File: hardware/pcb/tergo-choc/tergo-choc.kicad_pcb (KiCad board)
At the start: 2 copper layers, 161 x 108.8 mm, 131 parts, among them J1 TRRS, J2 Conn_01x04_Socket, J3 Conn_01x04_Socket, Q1 FDN335N, SW1 SW_Push, SW10 SW_Push, SW11 SW_Push, SW12 SW_Push, SW13 SW_Push, SW14 SW_Push, SW15 SW_Push, SW16 SW_Push, SW17 SW_Push, SW18 SW_Push, SW19 SW_Push, SW2 SW_Push, SW20 SW_Push, SW21 SW_Push, SW22 SW_Push, SW23 SW_Push, SW24 SW_Push, SW25 SW_Push, SW26 SW_Push, SW27 SW_Push, SW28 SW_Push, SW29 SW_Push, SW3 SW_Push, SW4 SW_Push, SW5 SW_Push, SW6 SW_Push, SW7 SW_Push, SW8 SW_Push, SW9 SW_Push, U1 Raspberry_Pi_Pico

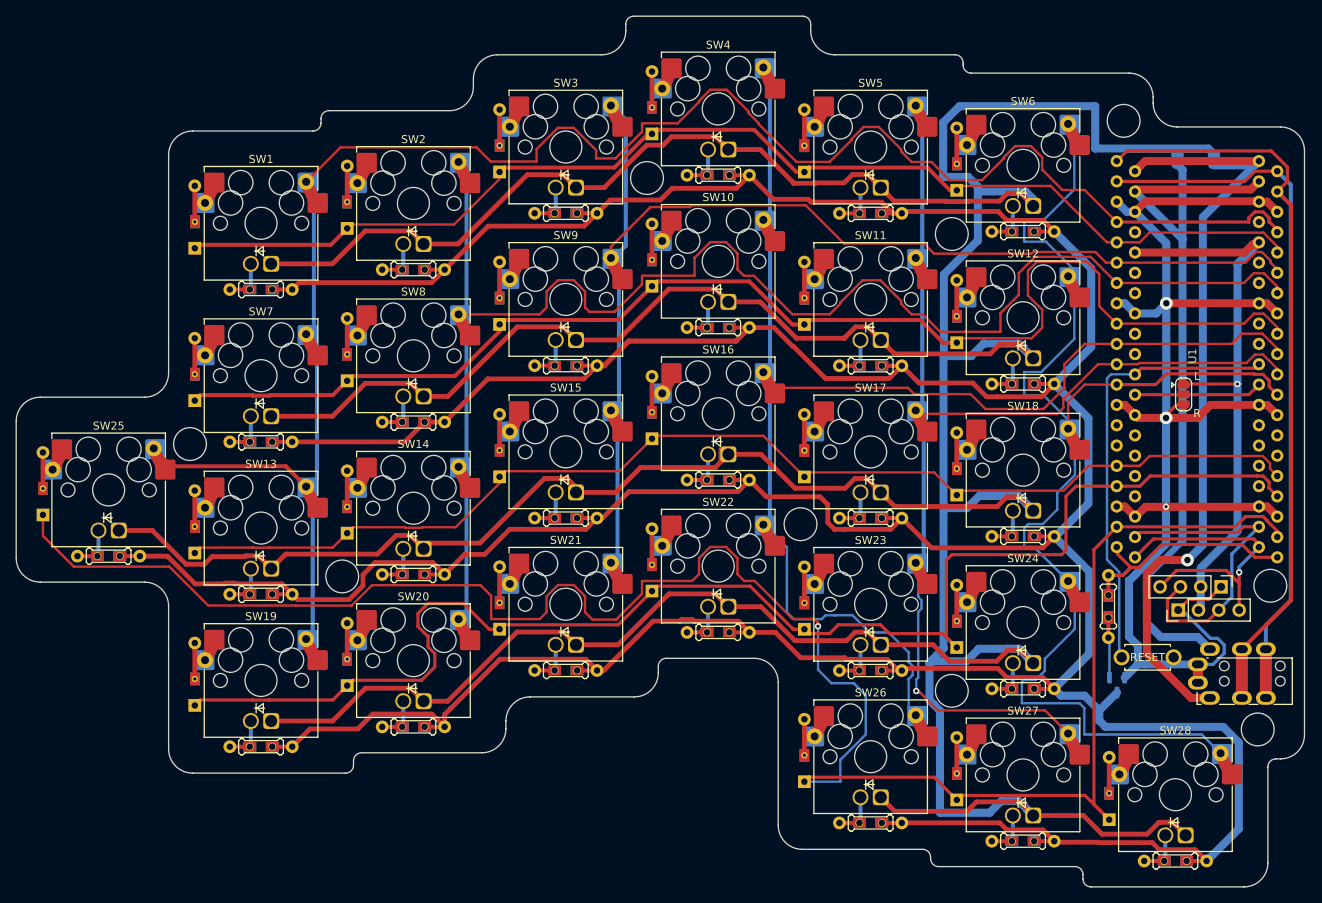
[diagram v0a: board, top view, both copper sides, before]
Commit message: wip
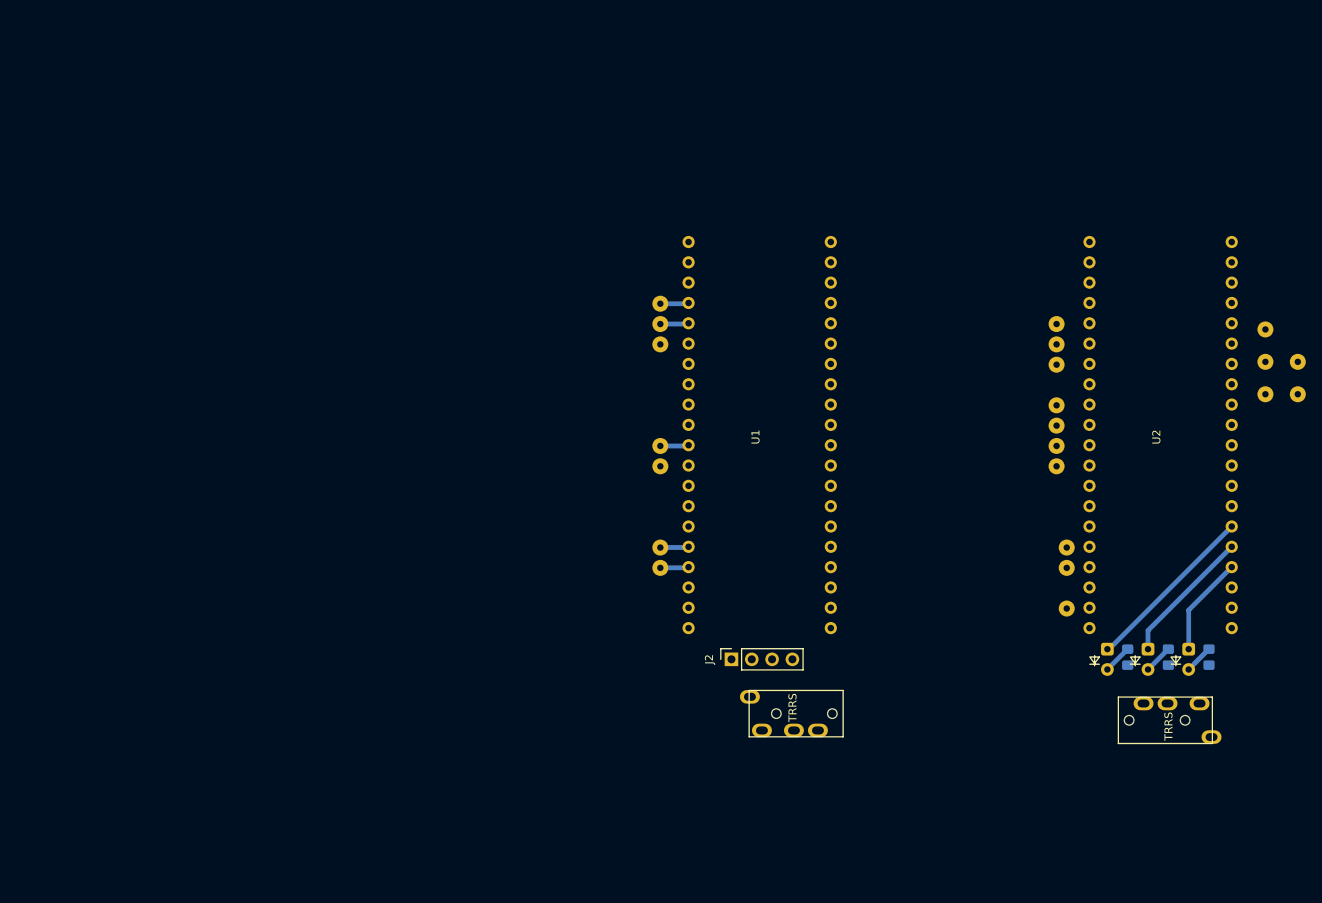
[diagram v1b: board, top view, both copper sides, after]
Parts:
- removed D1, D11, D12, D13, D14, D15, D16, D17, D18, D19, D2, D20, D21, D22, D23, D24, D25, D26, D27, D28, D3, D4, D5, D6, D7, D8, D9: D_Small, _tergo_lib:Diode-Hybrid-2sided
- removed D29, D30, D31, D32, D33, D34, D35, D36, D37, D38, D39, D40, D41, D42, D43, D44, D45, D46, D47, D48, D49, D50, D51, D52, D53, D54, D55, D56: LED_Small, _tergo_lib:LED_1.8mm
- removed H1, H2, H3, H4, H5, H6, H7, H8, H9: CaseHole, _tergo_lib:MountHole
- removed JP1: Jumper_3_Open, Jumper:SolderJumper-3_P1.3mm_Open_RoundedPad1.0x1.5mm
- removed JPL1, JPR2: Jumper_2_Open, Jumper:SolderJumper-2_P1.3mm_Open_RoundedPad1.0x1.5mm
- removed Q1: FDN335N, Package_TO_SOT_SMD:SOT-23
- removed R10, R11, R12, R13, R14, R15, R16, R17, R18, R19, R2, R20, R21, R22, R23, R24, R25, R26, R27, R28, R5, R6, R7, R8, R9: R_Small, _tergo_lib:Resistor-Hybrid-2sided
- removed R31: 10k, _tergo_lib:Resistor-Hybrid-2sided
- removed SW1, SW10, SW11, SW12, SW13, SW14, SW15, SW16, SW17, SW18, SW19, SW2, SW20, SW21, SW22, SW23, SW24, SW25, SW26, SW27, SW28, SW3, SW4, SW5, SW6, SW7, SW8, SW9: SW_Push, _tergo_lib:SW_Hotswap_Kailh_MX_Plated_mirrored2_1.00u
- removed SW29: SW_Push, _tergo_lib:ResetSW
- added D59: CL, _tergo_lib:LED_1.8mm, F.Cu at (184.2, 105.4)
- added D60: SL, _tergo_lib:LED_1.8mm, F.Cu at (189.2, 105.4)
- added J12: Conn_01x01_Socket, _tergo_lib:THT_PAD, F.Cu at (123.2, 61.0)
- added J13: Conn_01x01_Socket, _tergo_lib:THT_PAD, F.Cu at (123.2, 63.5)
- added J14: Conn_01x01_Socket, _tergo_lib:THT_PAD, F.Cu at (123.2, 66.0)
- added J15: Conn_01x01_Socket, _tergo_lib:THT_PAD, F.Cu at (198.8, 64.2)
- added J18: Conn_01x01_Socket, _tergo_lib:THT_PAD, F.Cu at (198.8, 68.2)
- added J19: Conn_01x01_Socket, _tergo_lib:THT_PAD, F.Cu at (198.8, 72.3)
- added J20: Conn_01x01_Socket, _tergo_lib:THT_PAD, F.Cu at (123.2, 78.7)
- added J21: Conn_01x01_Socket, _tergo_lib:THT_PAD, F.Cu at (123.2, 81.3)
- added J22: Conn_01x01_Socket, _tergo_lib:THT_PAD, F.Cu at (123.2, 91.4)
- added J23: Conn_01x01_Socket, _tergo_lib:THT_PAD, F.Cu at (123.2, 94.0)
- added J24: Conn_01x01_Socket, _tergo_lib:THT_PAD, F.Cu at (202.9, 68.2)
- added J25: Conn_01x01_Socket, _tergo_lib:THT_PAD, F.Cu at (202.9, 72.3)
- added J26: Conn_01x01_Socket, _tergo_lib:THT_PAD, F.Cu at (172.7, 63.5)
- added J27: Conn_01x01_Socket, _tergo_lib:THT_PAD, F.Cu at (172.7, 66.0)
- added J28: Conn_01x01_Socket, _tergo_lib:THT_PAD, F.Cu at (172.7, 68.6)
- added J29: Conn_01x01_Socket, _tergo_lib:THT_PAD, F.Cu at (172.7, 73.7)
- added J30: Conn_01x01_Socket, _tergo_lib:THT_PAD, F.Cu at (172.7, 76.2)
- added J31: Conn_01x01_Socket, _tergo_lib:THT_PAD, F.Cu at (172.7, 78.7)
- added J32: Conn_01x01_Socket, _tergo_lib:THT_PAD, F.Cu at (172.7, 81.3)
- added J33: Conn_01x01_Socket, _tergo_lib:THT_PAD, F.Cu at (174.0, 91.4)
- added J34: Conn_01x01_Socket, _tergo_lib:THT_PAD, F.Cu at (174.0, 94.0)
- added J35: Conn_01x01_Socket, _tergo_lib:THT_PAD, F.Cu at (174.0, 99.1)
- added U2: Raspberry_Pi_Pico, _tergo_lib:Raspberry_Pi_Pico, F.Cu at (185.7, 77.4)
- D10: value D_Small -> NL; footprint _tergo_lib:Diode-Hybrid-2sided -> _tergo_lib:LED_1.8mm
- J1: value TRRS -> TRRS_SOCKET; footprint _tergo_lib:MJ-4PP-9-mirrored -> _tergo_lib:MJ-4PP-9
- J2: footprint Connector_PinHeader_2.54mm:PinHeader_1x04_P2.54mm_Vertical -> Connector_PinSocket_2.54mm:PinSocket_1x04_P2.54mm_Vertical
- J3: value Conn_01x04_Socket -> TRRS_SOCKET; footprint Connector_PinHeader_2.54mm:PinHeader_1x04_P2.54mm_Vertical -> _tergo_lib:MJ-4PP-9
- R1, R3, R4: footprint _tergo_lib:Resistor-Hybrid-2sided -> Resistor_SMD:R_0805_2012Metric_Pad1.20x1.40mm_HandSolder; moved to B.Cu
- U1: footprint _tergo_lib:Raspberry_Pi_Pico_dual -> _tergo_lib:Raspberry_Pi_Pico
- moved R1 117.7 mm to (181.6, 105.1), turned to -90 degrees
- moved R3 93.5 mm to (186.7, 105.1), turned to -90 degrees
- moved R4 86.0 mm to (191.8, 105.1), turned to -90 degrees
- moved D10 76.1 mm to (179.1, 105.4), turned to 90 degrees
- moved J2 61.9 mm to (132.1, 105.4), turned to 90 degrees
- moved J1 56.1 mm to (146.2, 112.2)
- moved U1 54.5 mm to (135.6, 77.4)
- moved J3 15.8 mm to (180.3, 113.0)
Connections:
- D10 pad 1: /rowB -> Net-(D10-K)
- D10 pad 2: Net-(D10-A) -> /NUM_LOCK
- J1 pad B: /RX -> /VOUT_L
- J1 pad C: /TX -> /TX_L
- J2 pad 2: /3V3 -> /3V3_L
- R1 pad 1: Net-(D29-K) -> Net-(D10-K)
- R1 pad 2: /LEDOut -> GND
- R3 pad 2: /LEDOut -> GND
- R4 pad 2: /LEDOut -> GND
- U1 pad 10: /col3 -> /COL3_L
- U1 pad 11: /col4 -> /COL4_L
- U1 pad 12: /col5 -> /COL5_L
- U1 pad 16: /rowC -> /ROWC_L
- U1 pad 17: /rowD -> /ROWD_L
- U1 pad 19: /rowE -> /ROWE_L
- U1 pad 20: /LED -> unconnected-(U1-GP15-Pad20)
- U1 pad 29: Net-(JP1-C) -> /3V3_L
- U1 pad 30: /RST -> /RST_L
- U1 pad 36: /3V3 -> /3V3_L
- U1 pad 39: /Vin -> unconnected-(U1-Vin-Pad39)
- U1 pad 4: /col0 -> /COL0_L
- U1 pad 40: /Vout -> /VOUT_L
- U1 pad 5: /rowA -> /ROWA_L
- U1 pad 6: /col2 -> /COL2_L
- U1 pad 7: /col1 -> /COL1_L
- U1 pad 9: /rowB -> /ROWB_L
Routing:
- net /VCC_LED: track 698.5 -> 0.00 mm
- net /LEDOut: track 606.2 -> 0.00 mm
- net /rowE: track 255.9 -> 0.00 mm, vias 1 -> 0
- net /col0: track 230.9 -> 0.00 mm
- net /col1: track 193.1 -> 0.00 mm
- net GND: track 180.8 -> 0.00 mm, vias 3 -> 0
- net /rowD: track 177.8 -> 0.00 mm
- net /col3: track 170.4 -> 0.00 mm
- net /rowB: track 164.2 -> 0.00 mm
- net /col5: track 161.6 -> 0.00 mm
- net /col2: track 154.0 -> 0.00 mm
- net /rowA: track 150.7 -> 0.00 mm
- net /rowC: track 149.4 -> 0.00 mm
- net /col4: track 147.1 -> 0.00 mm, vias 1 -> 0
- net /Vout: track 101.4 -> 0.00 mm, vias 1 -> 0
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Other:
- board outline removed
- board text removed: "L"
- board text removed: "R"
